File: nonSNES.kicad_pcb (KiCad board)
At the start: 4 copper layers, 188 x 161.3 mm, 21 parts, among them J1 Jack-DC, P1 CASSETTE, P3 Conn_01x02_Male, T1 L_Coupled, U1 CPU, U12 L7805, U2 PPU1, U3 PPU2, U4 MS62256CL-10FC, U5 MS62256CL-10FC

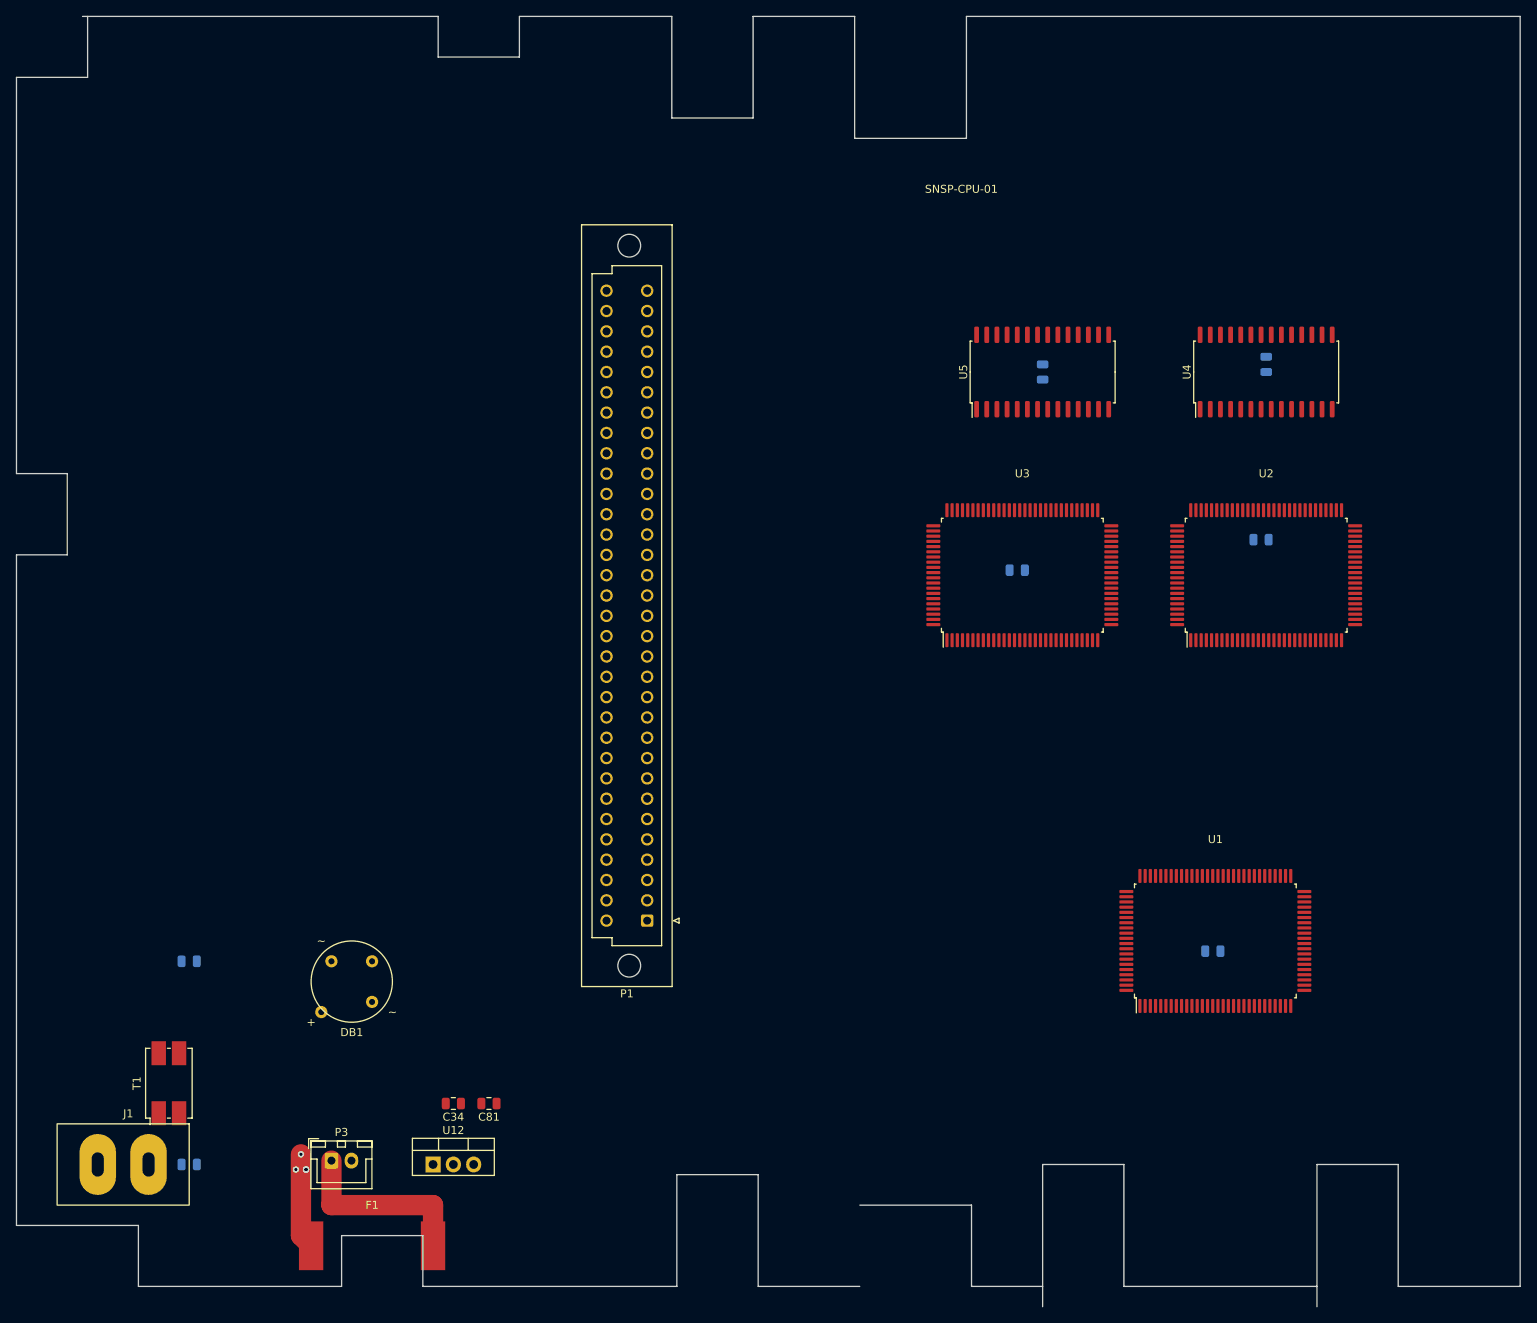
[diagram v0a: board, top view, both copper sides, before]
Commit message: add controller port
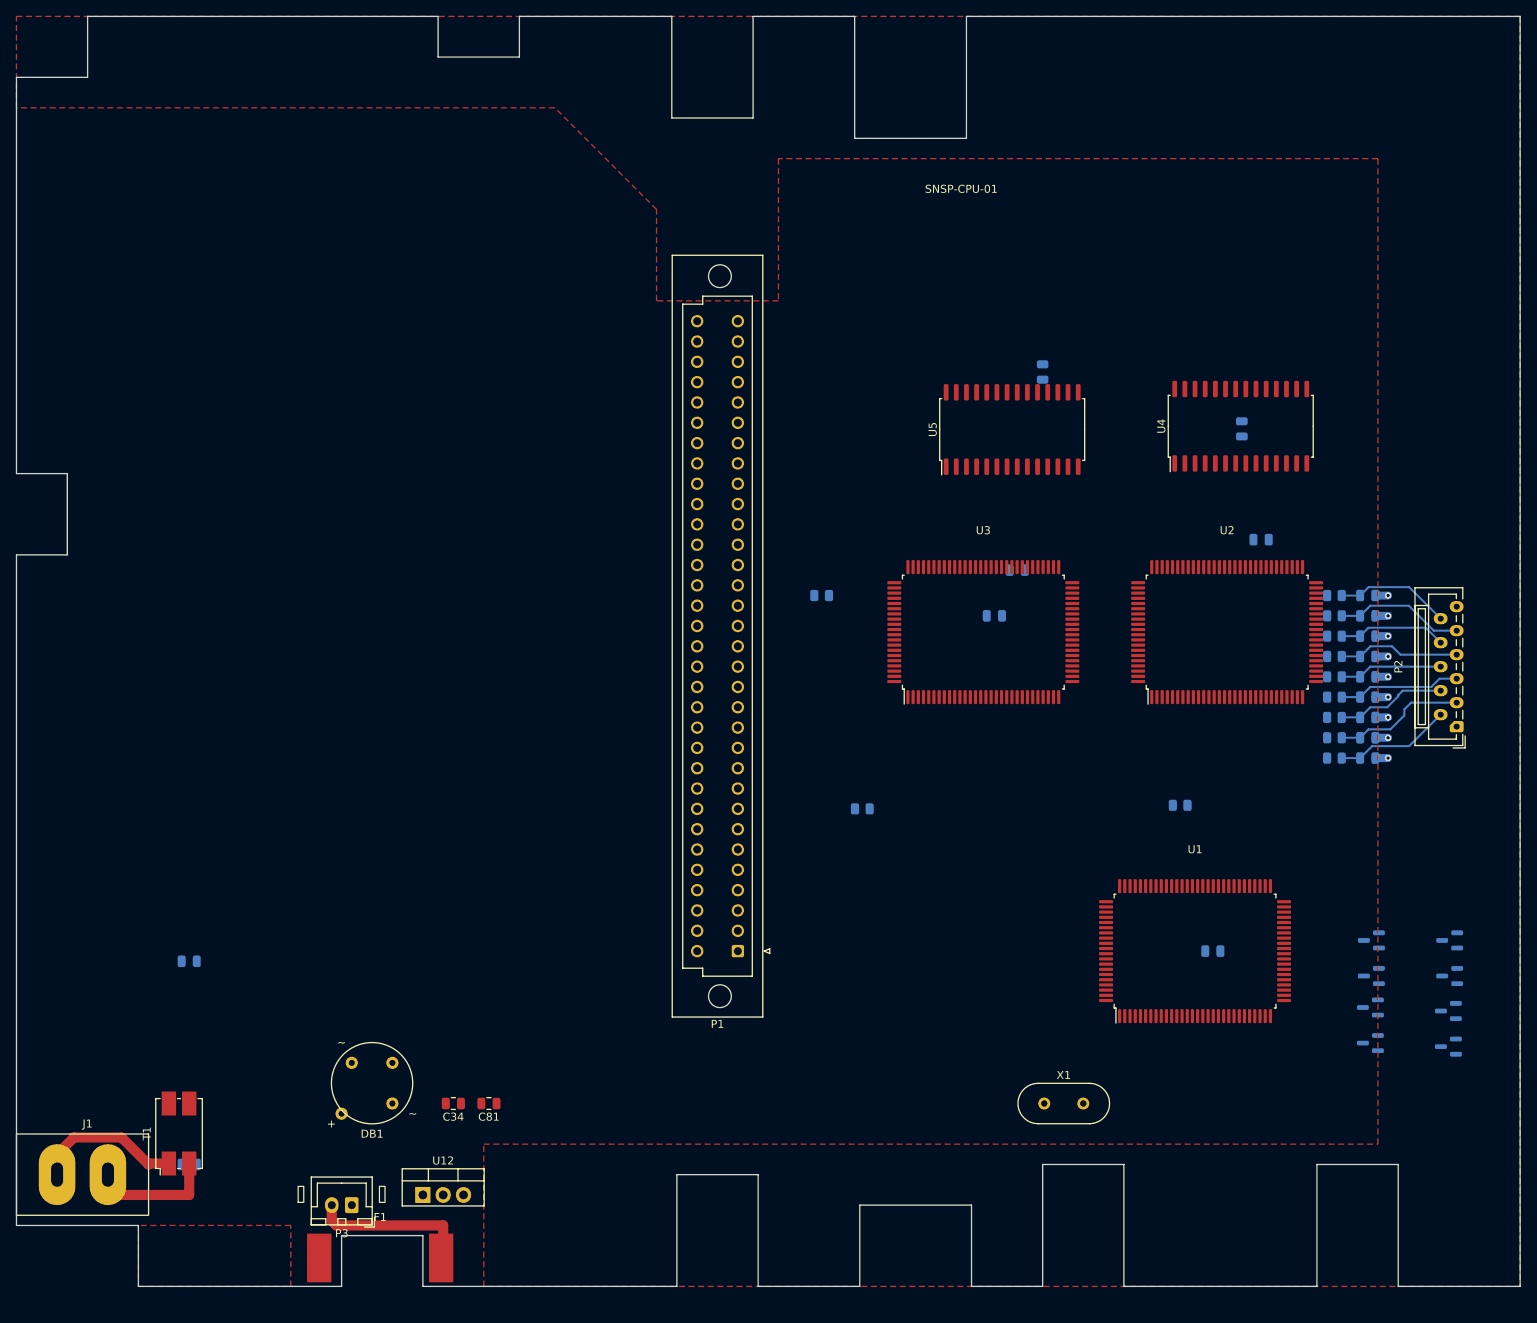
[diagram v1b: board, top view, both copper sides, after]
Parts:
- added C107: 0.01u, Capacitor_SMD:C_0805_2012Metric, B.Cu at (185.7, 128.3)
- added C35: 330p, Capacitor_SMD:C_0805_2012Metric, B.Cu at (232.4, 146.1)
- added C36: 330p, Capacitor_SMD:C_0805_2012Metric, B.Cu at (232.4, 143.5)
- added C37: 330p, Capacitor_SMD:C_0805_2012Metric, B.Cu at (232.4, 141.0)
- added C38: 330p, Capacitor_SMD:C_0805_2012Metric, B.Cu at (232.4, 138.4)
- added C39: 330p, Capacitor_SMD:C_0805_2012Metric, B.Cu at (232.4, 135.9)
- added C40: 330p, Capacitor_SMD:C_0805_2012Metric, B.Cu at (232.4, 133.3)
- added C41: 330p, Capacitor_SMD:C_0805_2012Metric, B.Cu at (232.4, 130.8)
- added C42: 330p, Capacitor_SMD:C_0805_2012Metric, B.Cu at (232.4, 128.3)
- added C43: 330p, Capacitor_SMD:C_0805_2012Metric, B.Cu at (232.4, 125.7)
- added DA10: D, Package_TO_SOT_SMD:SOT-23, B.Cu at (232.7, 181.7)
- added DA2: D, Package_TO_SOT_SMD:SOT-23, B.Cu at (242.6, 168.8)
- added DA3: D, Package_TO_SOT_SMD:SOT-23, B.Cu at (242.6, 173.3)
- added DA4: D, Package_TO_SOT_SMD:SOT-23, B.Cu at (242.5, 177.7)
- added DA5: D, Package_TO_SOT_SMD:SOT-23, B.Cu at (242.5, 182.1)
- added DA7: D, Package_TO_SOT_SMD:SOT-23, B.Cu at (232.9, 168.8)
- added DA8: D, Package_TO_SOT_SMD:SOT-23, B.Cu at (232.9, 173.3)
- added DA9: D, Package_TO_SOT_SMD:SOT-23, B.Cu at (232.7, 177.2)
- added P2: Conn_2Rows-11Pins, Connector_JST:JST_ZE_B11B-ZESK-D_1x11_P1.50mm_Vertical, F.Cu at (243.5, 142.1)
- added R78: 10k, Resistor_SMD:R_0805_2012Metric, B.Cu at (169.2, 152.4)
- added R80: 10k, Resistor_SMD:R_0805_2012Metric, B.Cu at (164.2, 125.7)
- added R82: 10k, Resistor_SMD:R_0805_2012Metric, B.Cu at (209.0, 151.9)
- added R83: 100, Resistor_SMD:R_0805_2012Metric, B.Cu at (228.2, 146.1)
- added R84: 100, Resistor_SMD:R_0805_2012Metric, B.Cu at (228.2, 143.5)
- added R85: 100, Resistor_SMD:R_0805_2012Metric, B.Cu at (228.2, 141.0)
- added R86: 100, Resistor_SMD:R_0805_2012Metric, B.Cu at (228.2, 138.4)
- added R87: 100, Resistor_SMD:R_0805_2012Metric, B.Cu at (228.2, 135.9)
- added R88: 100, Resistor_SMD:R_0805_2012Metric, B.Cu at (228.2, 133.3)
- added R89: 100, Resistor_SMD:R_0805_2012Metric, B.Cu at (228.2, 130.8)
- added R90: 100, Resistor_SMD:R_0805_2012Metric, B.Cu at (228.2, 128.3)
- added R91: 100, Resistor_SMD:R_0805_2012Metric, B.Cu at (228.2, 125.7)
- added X1: Crystal, Crystal:Crystal_HC49-4H_Vertical, F.Cu at (192.0, 189.2)
- moved DB1 13.0 mm to (108.0, 186.7)
- moved P1 12.0 mm to (153.7, 170.2)
- moved U2 8.62 mm to (214.8, 130.3)
- moved U3 8.62 mm to (184.4, 130.3)
- moved C97 8.62 mm to (216.7, 104.9)
- moved U5 8.14 mm to (188.0, 105.0)
- moved U4 7.49 mm to (216.5, 104.6)
- moved T1 6.42 mm to (83.8, 193.0)
- moved P3 6.11 mm to (105.4, 201.9), turned to 180 degrees
- moved J1 5.24 mm to (72.4, 198.1)
- moved U12 4.02 mm to (114.3, 200.7)
- moved U1 2.84 mm to (210.8, 170.2)
- moved F1 1.83 mm to (109.0, 208.5)
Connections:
- C34 pad 1: Net-(C34-Pad1) -> Net-(P3-Pin_1)
- F1 pad 2: Net-(F1-Pad2) -> Net-(P3-Pin_2)
- P3 pad 1: Net-(F1-Pad2) -> Net-(P3-Pin_1)
- P3 pad 2: Net-(C34-Pad1) -> Net-(P3-Pin_2)
- T1 pad 1: Net-(C30-Pad1) -> Net-(C30-Pad2)
- T1 pad 2: Net-(C30-Pad2) -> Net-(C30-Pad1)
- T1 pad 3: Net-(C31-Pad1) -> Net-(C31-Pad2)
- T1 pad 4: Net-(C31-Pad2) -> Net-(C31-Pad1)
- U1 pad 18: unconnected-(U1-Pad18) -> GND
- U1 pad 47: unconnected-(U1-Pad47) -> GND
- U1 pad 79: unconnected-(U1-Pad79) -> GND
- U1 pad 90: unconnected-(U1-Pad90) -> GND
- U12 pad 1: Net-(C34-Pad1) -> Net-(P3-Pin_1)
- U2 pad 22: unconnected-(U2-Pad22) -> GND
- U2 pad 28: unconnected-(U2-Pad28) -> /VDB0
- U2 pad 29: unconnected-(U2-Pad29) -> /VDB1
- U2 pad 30: unconnected-(U2-Pad30) -> /VDB2
- U2 pad 31: unconnected-(U2-Pad31) -> /VDB3
- U2 pad 32: unconnected-(U2-Pad32) -> /VDB4
- U2 pad 33: unconnected-(U2-Pad33) -> /VDB5
- U2 pad 34: unconnected-(U2-Pad34) -> /VDB6
- U2 pad 35: unconnected-(U2-Pad35) -> /VDB7
- U2 pad 37: unconnected-(U2-Pad37) -> /VDA0
- U2 pad 38: unconnected-(U2-Pad38) -> /VDA1
- U2 pad 39: unconnected-(U2-Pad39) -> /VDA2
- U2 pad 40: unconnected-(U2-Pad40) -> /VDA3
- U2 pad 41: unconnected-(U2-Pad41) -> /VDA4
- U2 pad 42: unconnected-(U2-Pad42) -> /VDA5
- U2 pad 43: unconnected-(U2-Pad43) -> /VDA6
- U2 pad 44: unconnected-(U2-Pad44) -> /VDA7
- U2 pad 45: unconnected-(U2-Pad45) -> GND
- U2 pad 47: unconnected-(U2-Pad47) -> /VA14
- U2 pad 48: unconnected-(U2-Pad48) -> /VAB13
- U2 pad 49: unconnected-(U2-Pad49) -> /VAB12
- U2 pad 50: unconnected-(U2-Pad50) -> /VAB11
- U2 pad 51: unconnected-(U2-Pad51) -> /VAB10
- U2 pad 52: unconnected-(U2-Pad52) -> /VAB9
- U2 pad 53: unconnected-(U2-Pad53) -> /VAB8
- U2 pad 54: unconnected-(U2-Pad54) -> /VAB7
- U2 pad 55: unconnected-(U2-Pad55) -> /VAB6
- U2 pad 56: unconnected-(U2-Pad56) -> /VAB5
- U2 pad 57: unconnected-(U2-Pad57) -> /VAB4
- U2 pad 58: unconnected-(U2-Pad58) -> /VAB3
- U2 pad 59: unconnected-(U2-Pad59) -> /VAB2
- U2 pad 60: unconnected-(U2-Pad60) -> /VAB1
- U2 pad 61: unconnected-(U2-Pad61) -> /VAB0
- U2 pad 63: unconnected-(U2-Pad63) -> /VAA13
- U2 pad 64: unconnected-(U2-Pad64) -> /VAA12
- U2 pad 65: unconnected-(U2-Pad65) -> /VAA11
- U2 pad 66: unconnected-(U2-Pad66) -> /VAA10
- U2 pad 67: unconnected-(U2-Pad67) -> /VAA9
- U2 pad 68: unconnected-(U2-Pad68) -> /VAA8
- U2 pad 69: unconnected-(U2-Pad69) -> /VAA7
- U2 pad 70: unconnected-(U2-Pad70) -> /VAA6
- U2 pad 71: unconnected-(U2-Pad71) -> /VAA5
- U2 pad 72: unconnected-(U2-Pad72) -> /VAA4
- U2 pad 73: unconnected-(U2-Pad73) -> /VAA3
- U2 pad 74: unconnected-(U2-Pad74) -> /VAA2
- U2 pad 75: unconnected-(U2-Pad75) -> /VAA1
- U2 pad 76: unconnected-(U2-Pad76) -> /VAA0
- U2 pad 77: unconnected-(U2-Pad77) -> GND
- U2 pad 96: unconnected-(U2-Pad96) -> GND
- U3 pad 16: unconnected-(U3-Pad16) -> GND
- U3 pad 30: unconnected-(U3-Pad30) -> GND
- U3 pad 35: unconnected-(U3-Pad35) -> GND
- U3 pad 51: unconnected-(U3-Pad51) -> /VDB0
- U3 pad 52: unconnected-(U3-Pad52) -> /VDB1
- U3 pad 53: unconnected-(U3-Pad53) -> /VDB2
- U3 pad 54: unconnected-(U3-Pad54) -> /VDB3
- U3 pad 55: unconnected-(U3-Pad55) -> /VDB4
- U3 pad 56: unconnected-(U3-Pad56) -> /VDB5
- U3 pad 57: unconnected-(U3-Pad57) -> /VDB6
- U3 pad 58: unconnected-(U3-Pad58) -> /VDB7
- U3 pad 60: unconnected-(U3-Pad60) -> /VDA0
- U3 pad 61: unconnected-(U3-Pad61) -> /VDA1
- U3 pad 62: unconnected-(U3-Pad62) -> /VDA2
- U3 pad 63: unconnected-(U3-Pad63) -> /VDA3
- U3 pad 64: unconnected-(U3-Pad64) -> /VDA4
- U3 pad 65: unconnected-(U3-Pad65) -> /VDA5
- U3 pad 66: unconnected-(U3-Pad66) -> /VDA6
- U3 pad 67: unconnected-(U3-Pad67) -> /VDA7
- U3 pad 68: unconnected-(U3-Pad68) -> GND
- U3 pad 69: unconnected-(U3-Pad69) -> /VDB0
- U3 pad 70: unconnected-(U3-Pad70) -> /VDB1
- U3 pad 71: unconnected-(U3-Pad71) -> /VDB2
- U3 pad 72: unconnected-(U3-Pad72) -> /VDB3
- U3 pad 73: unconnected-(U3-Pad73) -> /VDB4
- U3 pad 74: unconnected-(U3-Pad74) -> /VDB5
- U3 pad 75: unconnected-(U3-Pad75) -> /VDB6
- U3 pad 76: unconnected-(U3-Pad76) -> /VDB7
- U3 pad 90: unconnected-(U3-Pad90) -> GND
- U3 pad 91: unconnected-(U3-Pad91) -> GND
- U3 pad 92: unconnected-(U3-Pad92) -> GND
- U3 pad 93: unconnected-(U3-Pad93) -> GND
- U3 pad 94: unconnected-(U3-Pad94) -> VCC
- U3 pad 99: unconnected-(U3-Pad99) -> GND
- U4 pad 1: unconnected-(U4-Pad1) -> /VA14
- U4 pad 10: unconnected-(U4-Pad10) -> /VAB0
- U4 pad 11: /D0 -> /VDB0
- U4 pad 12: /D1 -> /VDB1
- U4 pad 13: /D2 -> /VDB2
- U4 pad 15: /D3 -> /VDB3
- U4 pad 16: /D4 -> /VDB4
- U4 pad 17: /D5 -> /VDB5
- U4 pad 18: /D6 -> /VDB6
- U4 pad 19: /D7 -> /VDB7
- U4 pad 2: unconnected-(U4-Pad2) -> /VAB12
- U4 pad 21: unconnected-(U4-Pad21) -> /VAB10
- U4 pad 23: unconnected-(U4-Pad23) -> /VAB11
- U4 pad 24: unconnected-(U4-Pad24) -> /VAB9
- U4 pad 25: unconnected-(U4-Pad25) -> /VAB8
- U4 pad 26: unconnected-(U4-Pad26) -> /VAB13
- U4 pad 3: unconnected-(U4-Pad3) -> /VAB7
- U4 pad 4: unconnected-(U4-Pad4) -> /VAB6
- U4 pad 5: unconnected-(U4-Pad5) -> /VAB5
- U4 pad 6: unconnected-(U4-Pad6) -> /VAB4
- U4 pad 7: unconnected-(U4-Pad7) -> /VAB3
- U4 pad 8: unconnected-(U4-Pad8) -> /VAB2
- U4 pad 9: unconnected-(U4-Pad9) -> /VAB1
- U5 pad 1: unconnected-(U5-Pad1) -> /VA14
- U5 pad 10: unconnected-(U5-Pad10) -> /VAA0
- U5 pad 11: /D0 -> /VDA0
- U5 pad 12: /D1 -> /VDA1
- U5 pad 13: /D2 -> /VDA2
- U5 pad 15: /D3 -> /VDA3
- U5 pad 16: /D4 -> /VDA4
- U5 pad 17: /D5 -> /VDA5
- U5 pad 18: /D6 -> /VDA6
- U5 pad 19: /D7 -> /VDA7
- U5 pad 2: unconnected-(U5-Pad2) -> /VAA12
- U5 pad 21: unconnected-(U5-Pad21) -> /VAA10
- U5 pad 23: unconnected-(U5-Pad23) -> /VAA11
- U5 pad 24: unconnected-(U5-Pad24) -> /VAA9
- U5 pad 25: unconnected-(U5-Pad25) -> /VAA8
- U5 pad 26: unconnected-(U5-Pad26) -> /VAA13
- U5 pad 3: unconnected-(U5-Pad3) -> /VAA7
- U5 pad 4: unconnected-(U5-Pad4) -> /VAA6
- U5 pad 5: unconnected-(U5-Pad5) -> /VAA5
- U5 pad 6: unconnected-(U5-Pad6) -> /VAA4
- U5 pad 7: unconnected-(U5-Pad7) -> /VAA3
- U5 pad 8: unconnected-(U5-Pad8) -> /VAA2
- U5 pad 9: unconnected-(U5-Pad9) -> /VAA1
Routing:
- net Net-(F1-Pad2): track 23.3 -> 0.00 mm
- net Net-(P3-Pin_2): track 0.00 -> 20.3 mm
- net Net-(C30-Pad2): track 0.00 -> 18.8 mm
- net Net-(C30-Pad1): track 0.00 -> 16.6 mm
- net Net-(P2-Pin_3): track 0.00 -> 16.6 mm
- net Net-(P2-Pin_9): track 0.00 -> 16.2 mm
- net Net-(P2-Pin_5): track 0.00 -> 15.3 mm
- net Net-(P2-Pin_7): track 0.00 -> 15.3 mm
- net Net-(P2-Pin_2): track 0.00 -> 14.6 mm
- net Net-(P2-Pin_10): track 0.00 -> 14.4 mm
- net GND: track 0.00 -> 14.3 mm, vias 0 -> 9
- net Net-(P2-Pin_4): track 0.00 -> 13.8 mm
- net Net-(P2-Pin_8): track 0.00 -> 13.6 mm
- net Net-(P2-Pin_6): track 0.00 -> 12.9 mm
- net Net-(DB1-+): track 12.0 -> 0.00 mm, vias 4 -> 0
- added copper zone on F.Cu, net GND
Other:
- board size 188 x 161.3 mm -> 188 x 158.8 mm
